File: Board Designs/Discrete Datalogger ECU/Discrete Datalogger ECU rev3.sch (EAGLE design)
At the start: 8 parts, among them X1 CONNECTOR-4

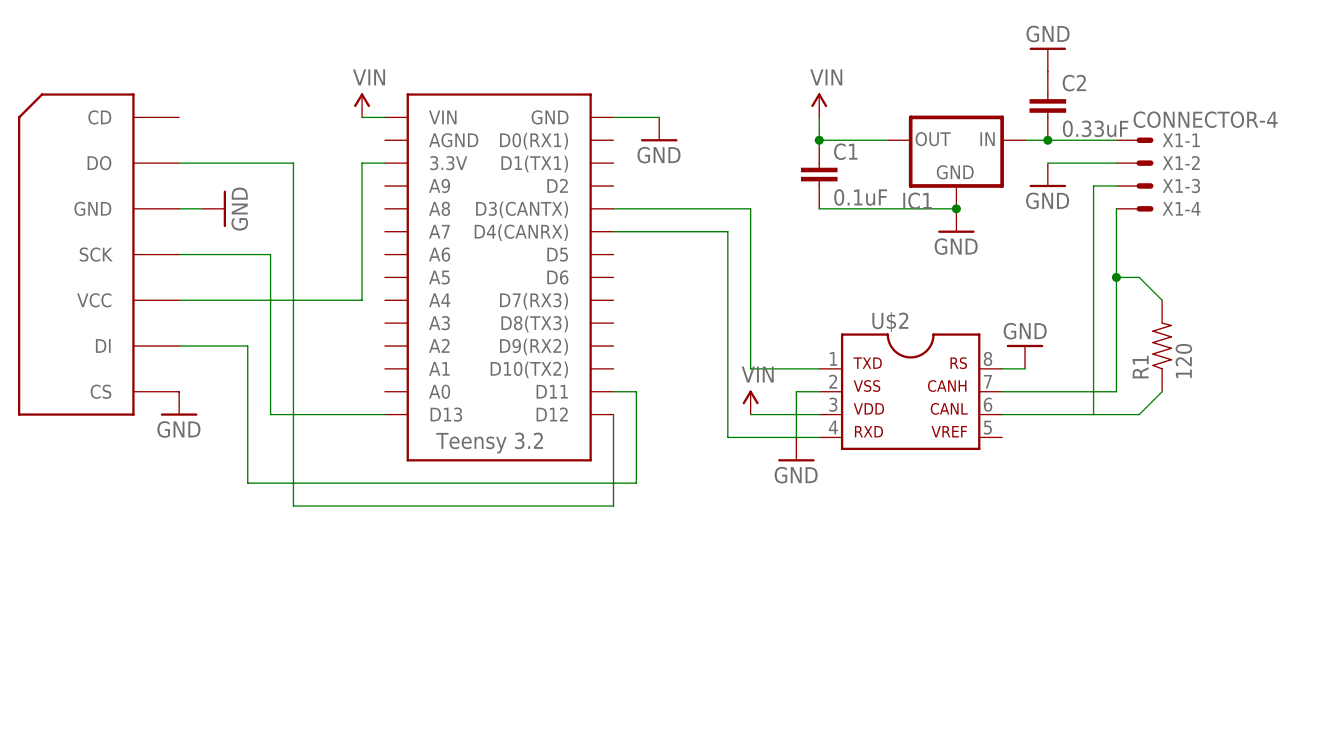
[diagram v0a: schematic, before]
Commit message: CAN Datalogger board rev3 - manufacture at JLC
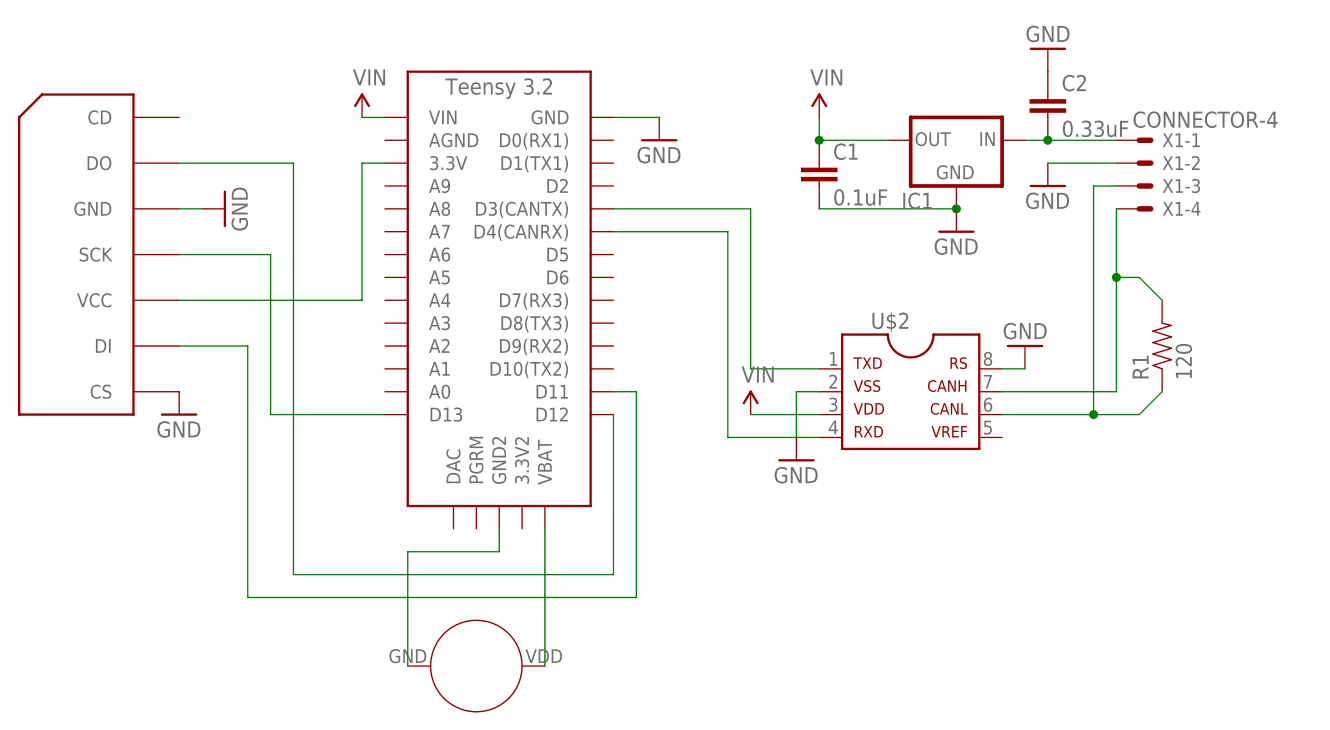
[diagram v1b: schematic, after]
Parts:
- added U$4: COIN-CELL-HOLDER, HyTechDevices:COIN-CELL-HOLDER
- U$1: value TEENSY_3.2_SIMPLE -> TEENSY_3.2_EXT; device HyTechDevices:TEENSY_3.2_SIMPLE -> HyTechDevices:TEENSY_3.2_EXT
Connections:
- new net N$1: U$1.VBAT, U$4.VDD
- new net N$2: U$1.GND2, U$4.GND
